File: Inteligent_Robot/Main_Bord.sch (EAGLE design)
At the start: 88 parts, among them CN5 DF11-4DS-2C, CN6 DF11-4DS-2C, CN7 IL-G_ST_4, CN8 IL-G_ST_4, IC1 TWE-001L-IP, IC2 LTC2862A, IC5 A4988, IC7 A4988

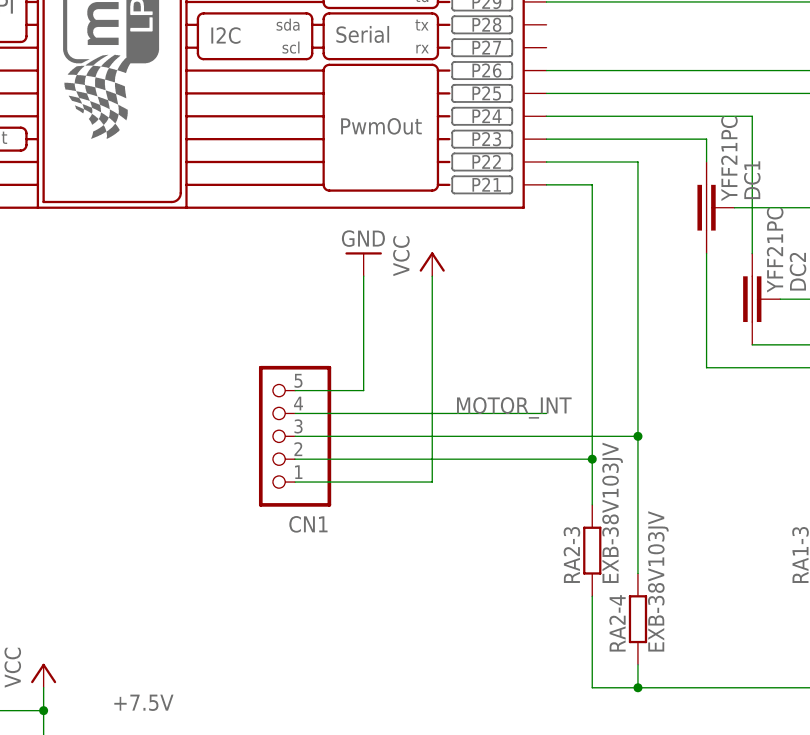
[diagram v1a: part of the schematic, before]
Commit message: Refime pisitions
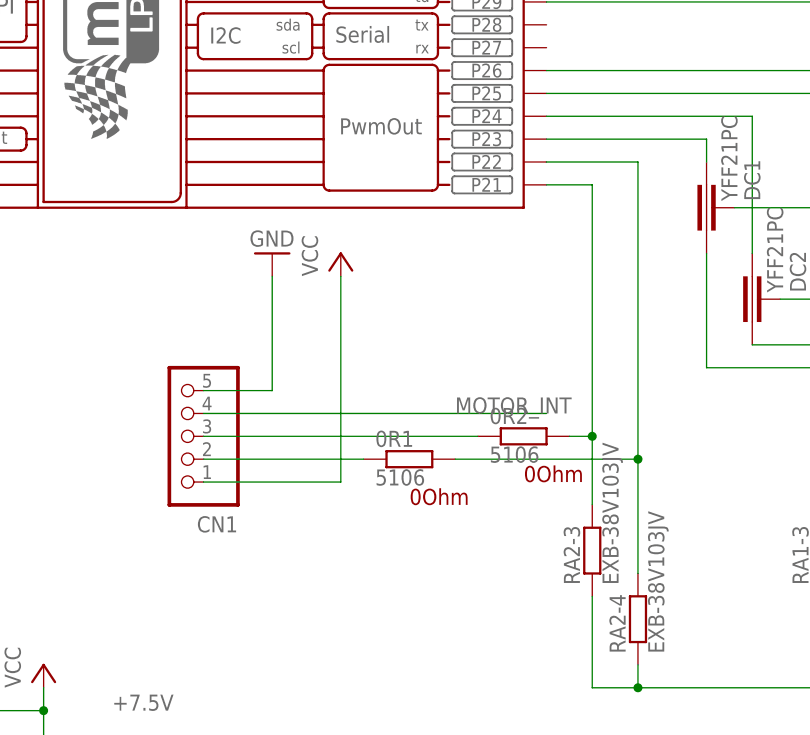
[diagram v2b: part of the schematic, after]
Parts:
- added 0R1, 0R2: 5106, Keystone:5106
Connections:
- new net N$10: 0R2.2, CN1.3
- new net N$11: 0R1.2, CN1.2
- net N$1: now also 0R2.1; no longer CN1.2
- net N$2: now also 0R1.1; no longer CN1.3
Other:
- moved on the sheet: CN1
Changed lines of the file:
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@@
 <layer number="59" name="tCarbon" color="7" fill="1" visible="no" active="no"/>
 <layer number="60" name="bCarbon" color="7" fill="1" visible="no" active="no"/>
+<layer number="88" name="SimResults" color="9" fill="1" visible="yes" active="yes"/>
+<layer number="89" name="SimProbes" color="9" fill="1" visible="yes" active="yes"/>
 <layer number="90" name="Modules" color="5" fill="1" visible="yes" active="yes"/>
 <layer number="91" name="Nets" color="2" fill="1" visible="yes" active="yes"/>
@@
 <part name="C10" library="Murata" deviceset="GMR31" device=""/>
 <part name="GND8" library="supply1" library_urn="urn:adsk.eagle:library:371" deviceset="GND" device=""/>
+<part name="0R1" library="Keystone" deviceset="5106" device=""/>
+<part name="0R2" library="Keystone" deviceset="5106" device=""/>
 </parts>
 <sheets>
@@
 <instance part="KIT1" gate="KIT" x="40.64" y="60.96"/>
 <instance part="IC1" gate="G$1" x="218.44" y="53.34" rot="MR0"/>
-<instance part="CN1" gate="G$1" x="60.96" y="7.62" rot="R180"/>
+<instance part="CN1" gate="G$1" x="50.8" y="7.62" rot="R180"/>
 <instance part="CN3" gate="G$1" x="43.18" y="-99.06"/>
 <instance part="GND2" gate="1" x="243.84" y="-25.4" rot="MR0"/>
@@
 <instance part="+3.3V1" gate="G$1" x="-43.18" y="142.24"/>
 <instance part="GND5" gate="1" x="185.42" y="20.32" rot="MR0"/>
-<instance part="P+2" gate="VCC" x="76.2" y="27.94"/>
-<instance part="GND6" gate="1" x="68.58" y="27.94" rot="MR180"/>
+<instance part="P+2" gate="VCC" x="66.04" y="27.94"/>
+<instance part="GND6" gate="1" x="58.42" y="27.94" rot="MR180"/>
 <instance part="P+5" gate="VCC" x="-10.16" y="-17.78"/>
 <instance part="GND11" gate="1" x="-15.24" y="-53.34"/>
@@
 <instance part="C10" gate="G$1" x="193.04" y="-114.3"/>
 <instance part="GND8" gate="1" x="-12.7" y="76.2"/>
+<instance part="0R1" gate="G$1" x="73.66" y="5.08"/>
+<instance part="0R2" gate="G$1" x="86.36" y="7.62"/>
 </instances>
 <busses>
@@
 <segment>
 <pinref part="CN1" gate="G$1" pin="5"/>
-<wire x1="60.96" y1="12.7" x2="68.58" y2="12.7" width="0.1524" layer="91"/>
+<wire x1="50.8" y1="12.7" x2="58.42" y2="12.7" width="0.1524" layer="91"/>
 <pinref part="GND6" gate="1" pin="GND"/>
-<wire x1="68.58" y1="12.7" x2="68.58" y2="25.4" width="0.1524" layer="91"/>
+<wire x1="58.42" y1="12.7" x2="58.42" y2="25.4" width="0.1524" layer="91"/>
 </segment>
 <segment>
@@
 <segment>
 <pinref part="CN1" gate="G$1" pin="1"/>
-<wire x1="60.96" y1="2.54" x2="76.2" y2="2.54" width="0.1524" layer="91"/>
+<wire x1="50.8" y1="2.54" x2="66.04" y2="2.54" width="0.1524" layer="91"/>
 <pinref part="P+2" gate="VCC" pin="VCC"/>
-<wire x1="76.2" y1="2.54" x2="76.2" y2="25.4" width="0.1524" layer="91"/>
+<wire x1="66.04" y1="2.54" x2="66.04" y2="25.4" width="0.1524" layer="91"/>
 </segment>
 <segment>
@@
 <pinref part="KIT1" gate="KIT" pin="P21"/>
 <wire x1="88.9" y1="35.56" x2="93.98" y2="35.56" width="0.1524" layer="91"/>
-<wire x1="93.98" y1="35.56" x2="93.98" y2="5.08" width="0.1524" layer="91"/>
-<pinref part="CN1" gate="G$1" pin="2"/>
-<wire x1="60.96" y1="5.08" x2="93.98" y2="5.08" width="0.1524" layer="91"/>
-<junction x="93.98" y="5.08"/>
+<wire x1="93.98" y1="35.56" x2="93.98" y2="7.62" width="0.1524" layer="91"/>
 <pinref part="RA2" gate="-3" pin="1"/>
-<wire x1="93.98" y1="0" x2="93.98" y2="5.08" width="0.1524" layer="91"/>
+<pinref part="0R2" gate="G$1" pin="1"/>
+<wire x1="93.98" y1="7.62" x2="93.98" y2="0" width="0.1524" layer="91"/>
+<wire x1="91.44" y1="7.62" x2="93.98" y2="7.62" width="0.1524" layer="91"/>
+<junction x="93.98" y="7.62"/>
 </segment>
 </net>
@@
 <pinref part="KIT1" gate="KIT" pin="P22"/>
 <wire x1="88.9" y1="38.1" x2="99.06" y2="38.1" width="0.1524" layer="91"/>
-<wire x1="99.06" y1="38.1" x2="99.06" y2="7.62" width="0.1524" layer="91"/>
-<pinref part="CN1" gate="G$1" pin="3"/>
-<wire x1="99.06" y1="7.62" x2="99.06" y2="-7.62" width="0.1524" layer="91"/>
-<wire x1="60.96" y1="7.62" x2="99.06" y2="7.62" width="0.1524" layer="91"/>
-<junction x="99.06" y="7.62"/>
+<wire x1="99.06" y1="38.1" x2="99.06" y2="5.08" width="0.1524" layer="91"/>
 <pinref part="RA2" gate="-4" pin="1"/>
+<pinref part="0R1" gate="G$1" pin="1"/>
+<wire x1="99.06" y1="5.08" x2="99.06" y2="-7.62" width="0.1524" layer="91"/>
+<wire x1="78.74" y1="5.08" x2="99.06" y2="5.08" width="0.1524" layer="91"/>
+<junction x="99.06" y="5.08"/>
 </segment>
 </net>
@@
 <segment>
 <pinref part="CN1" gate="G$1" pin="4"/>
-<wire x1="60.96" y1="10.16" x2="88.9" y2="10.16" width="0.1524" layer="91"/>
+<wire x1="50.8" y1="10.16" x2="88.9" y2="10.16" width="0.1524" layer="91"/>
 <label x="78.74" y="10.16" size="1.778" layer="95"/>
 </segment>
@@
 </segment>
 </net>
+<net name="N$10" class="0">
+<segment>
+<pinref part="0R2" gate="G$1" pin="2"/>
+<pinref part="CN1" gate="G$1" pin="3"/>
+<wire x1="50.8" y1="7.62" x2="81.28" y2="7.62" width="0.1524" layer="91"/>
+</segment>
+</net>
+<net name="N$11" class="0">
+<segment>
+<pinref part="0R1" gate="G$1" pin="2"/>
+<pinref part="CN1" gate="G$1" pin="2"/>
+<wire x1="50.8" y1="5.08" x2="68.58" y2="5.08" width="0.1524" layer="91"/>
+</segment>
+</net>
